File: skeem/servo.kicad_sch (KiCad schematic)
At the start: 9 parts, among them J10 Conn_01x03_Pin, U2 74HCT4851, U6 74HCT4851, U7 74LVC2G53

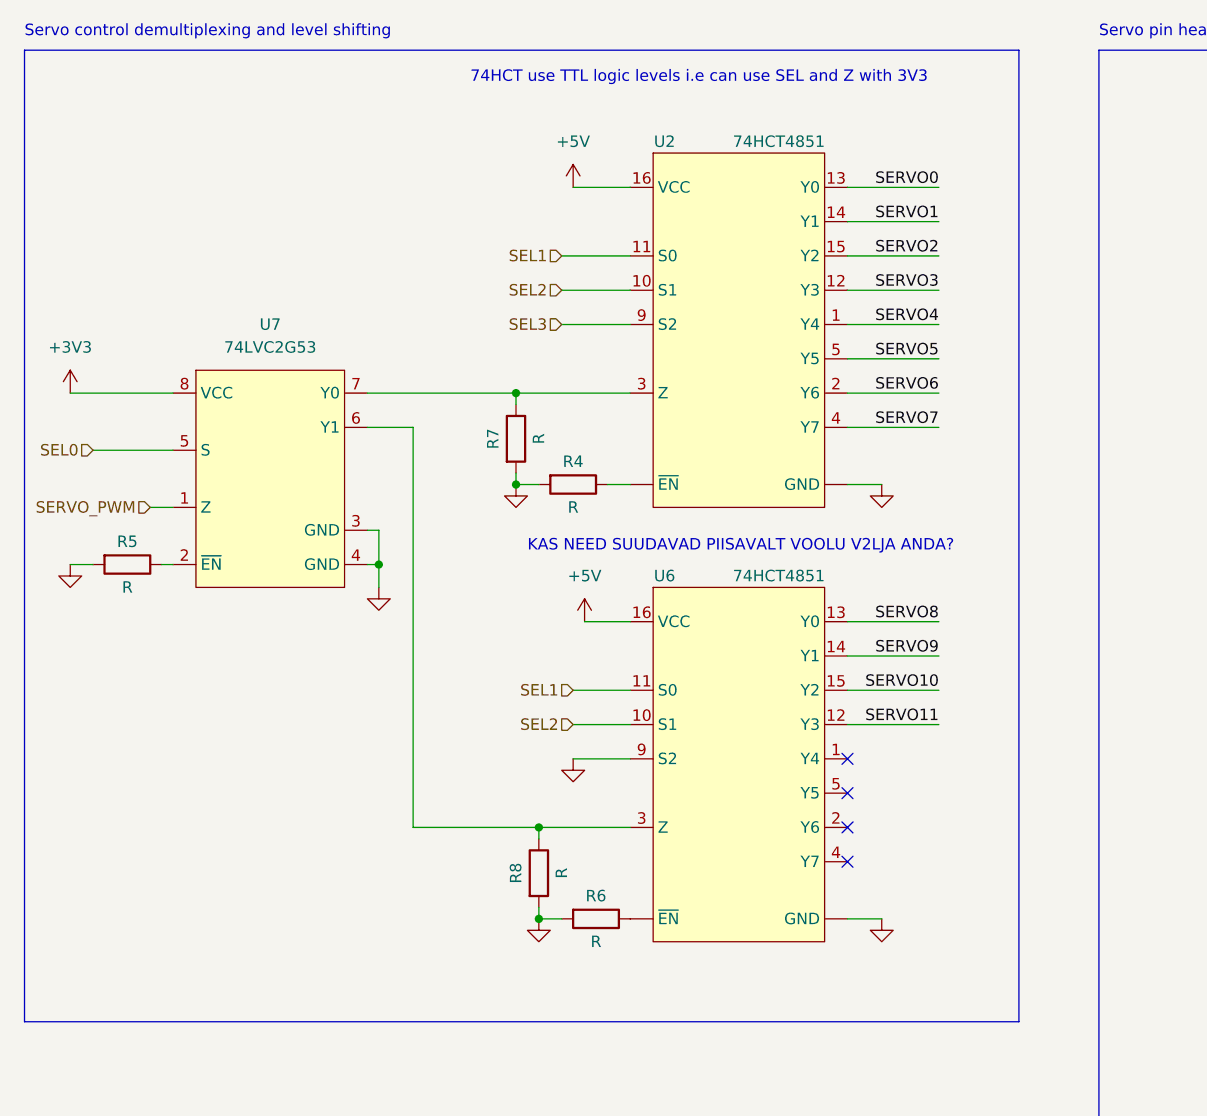
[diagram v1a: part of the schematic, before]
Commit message: power mgmt
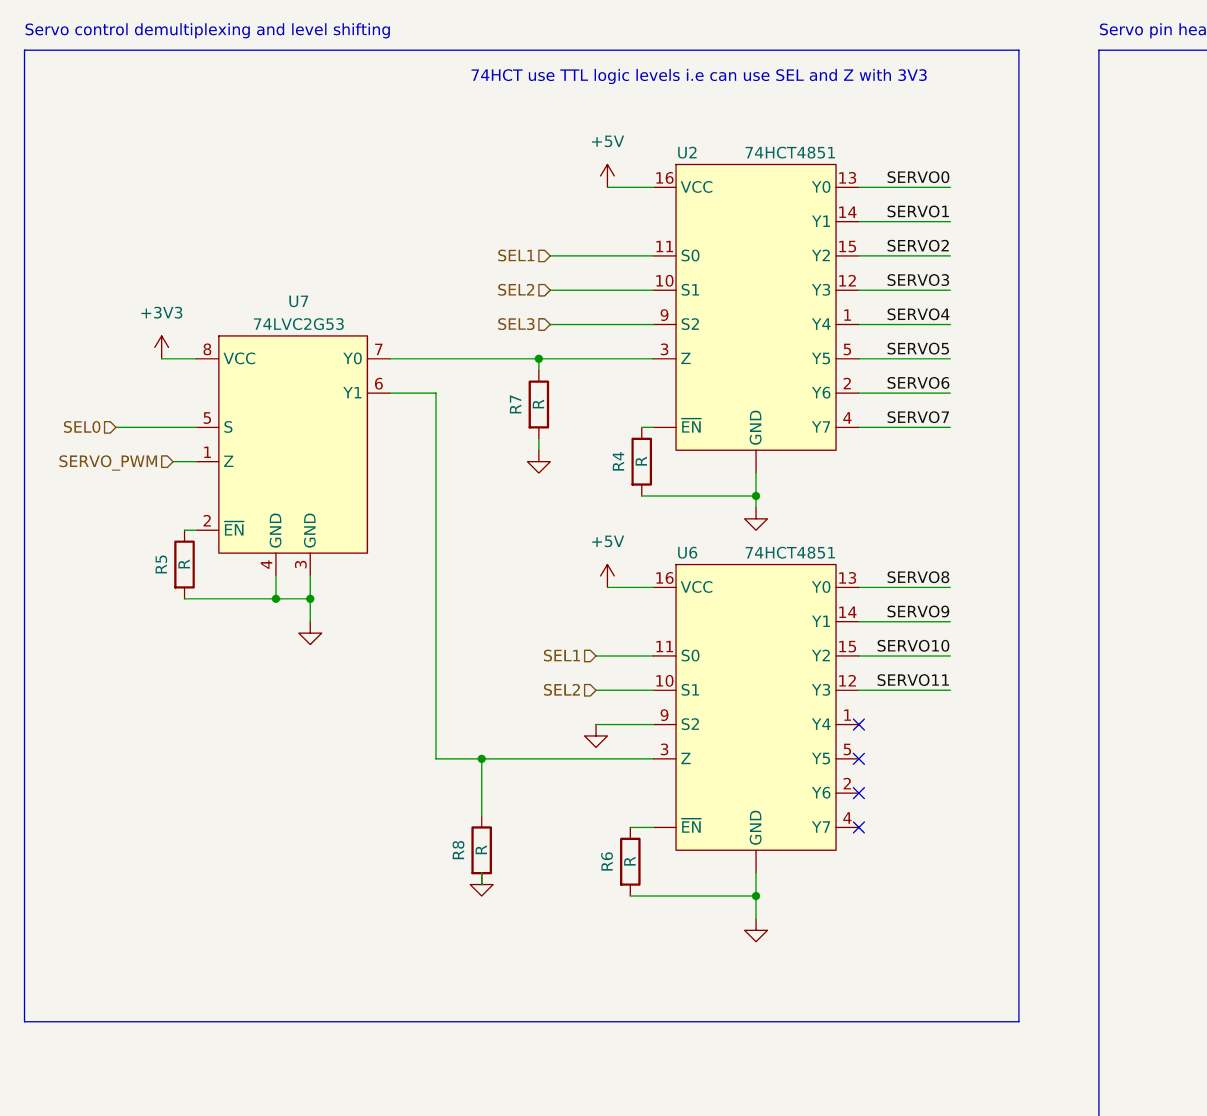
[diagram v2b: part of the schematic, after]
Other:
- note removed: "KAS NEED SUUDAVAD PIISAVALT VOOLU V2LJA ANDA?"
- moved on the sheet: R4, R5, R6, R7, R8, U2, U6, U7
